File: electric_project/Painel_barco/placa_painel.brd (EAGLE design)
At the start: 60 x 100 mm, 15 parts, among them IC1 7805TV

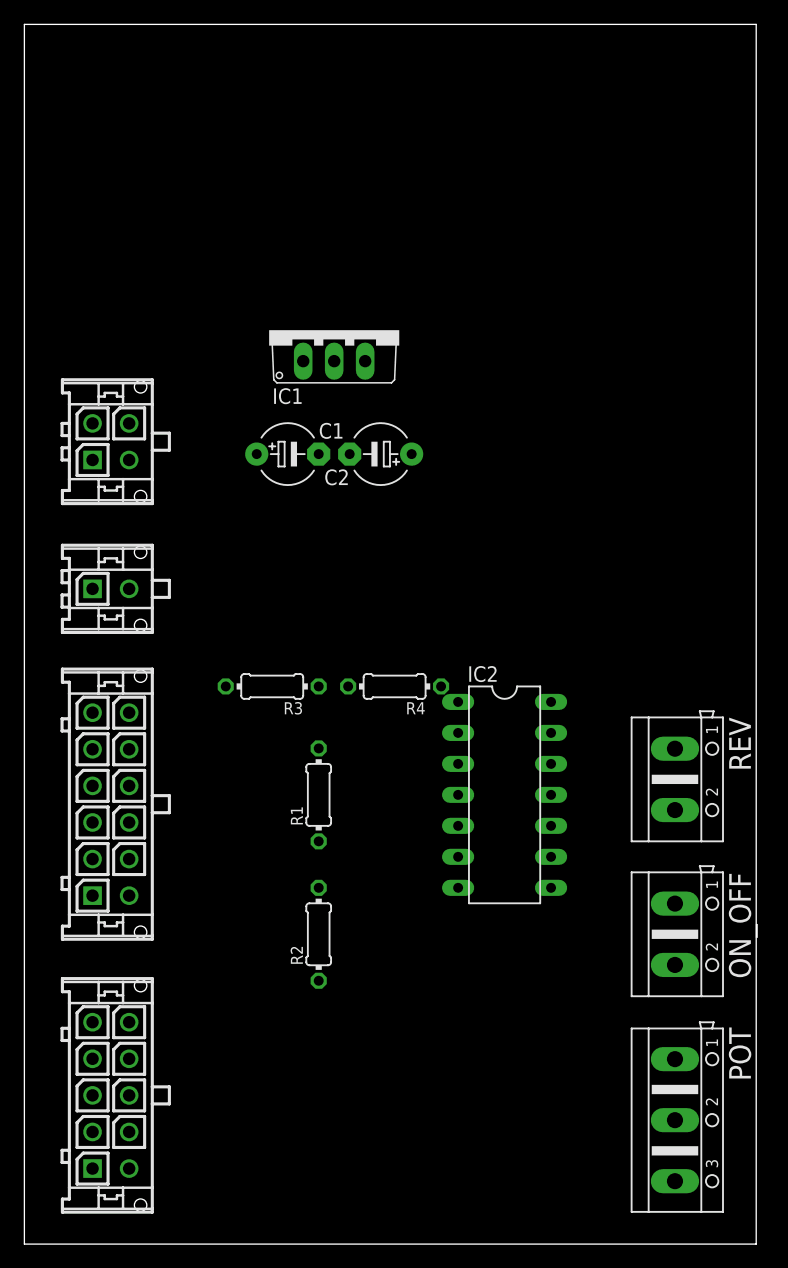
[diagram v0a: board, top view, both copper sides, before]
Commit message: up
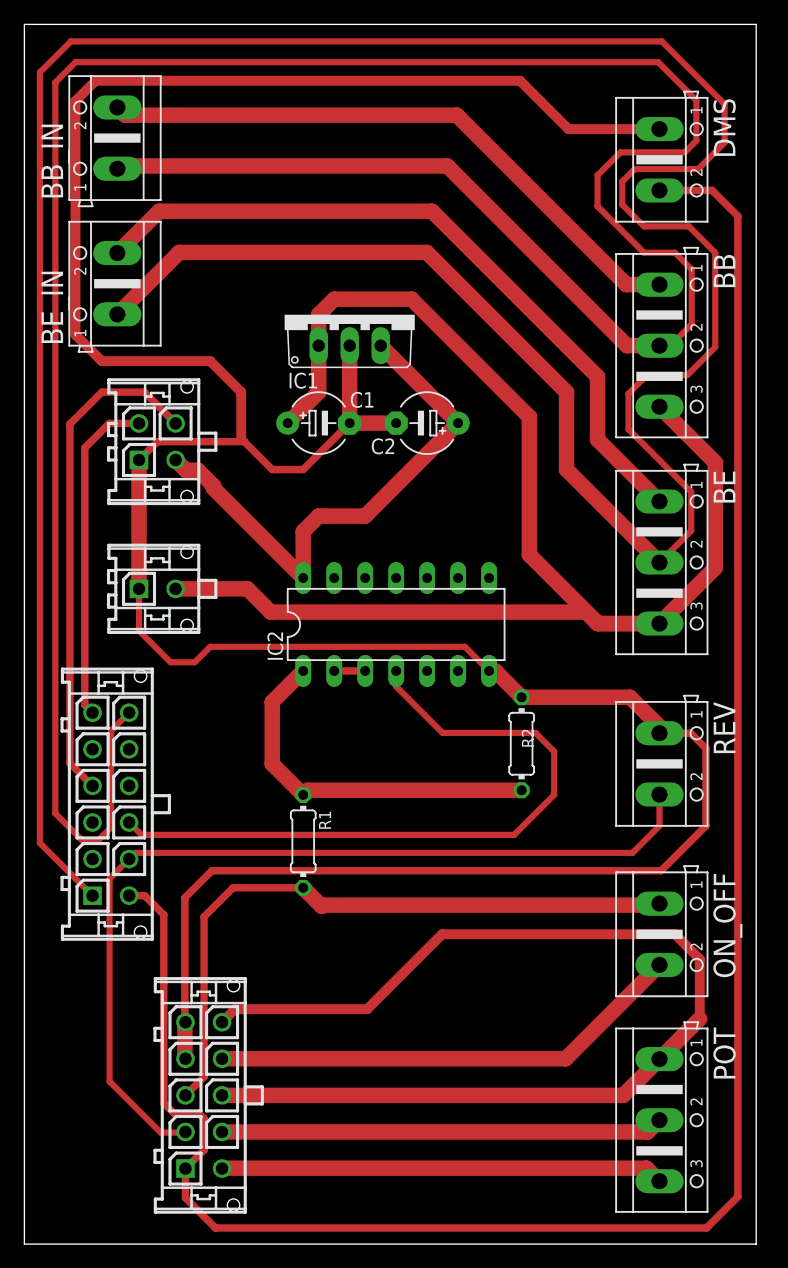
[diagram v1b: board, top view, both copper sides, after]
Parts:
- removed R3, R4: (no value), rcl:0204/7
- removed X2: (no value), con-molex-micro-fit-3_0:43045-1012
- added BB, BE: (no value), con-ptr500:AK500/3
- added BB_IN, BE_IN, DMS: (no value), con-ptr500:AK500/2
- added MOTOR_CON: (no value), con-molex-micro-fit-3_0:43045-1012
- moved R2 22.8 mm to (40.8, 41.0), turned to 270 degrees
- moved IC2 16.6 mm to (30.5, 50.8), turned to 0 degrees
- moved C2 4.58 mm to (33.0, 67.3)
- moved R1 4.02 mm to (22.9, 33.0), turned to 270 degrees
- moved X3 3.81 mm to (9.40, 53.7)
- moved X7 3.81 mm to (9.40, 65.8)
- moved C1 3.59 mm to (24.1, 67.3)
- moved IC1 1.80 mm to (26.7, 76.2)
- moved REV 1.80 mm to (52.1, 39.4)
- moved ON_OFF 1.27 mm to (52.1, 25.4)
- moved POT 1.27 mm to (52.1, 10.2)
- renumbered X1 to TELE_CON
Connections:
- removed net BB_IN: TELE_CON.P$12
- removed net BE_IN: TELE_CON.P$1
- removed net DMS_IN: TELE_CON.P$7
- removed net N$8: R3.1, R4.2
- new net BB_AUTO: BB.1, BB_IN.2
- new net BB_RET: BB.2, BB_IN.1, TELE_CON.P$12
- new net BE_AUTO: BE.1, BE_IN.2
- new net BE_RET: BE.2, BE_IN.1, TELE_CON.P$1
- new net WHITE_DMS: DMS.2, MOTOR_CON.P$1, TELE_CON.P$7
- net 21: now also X7.P$4; no longer X7.P$3
- net 22: now also X7.P$2; no longer X7.P$4
- net BLACK_GND: now also MOTOR_CON.P$10, MOTOR_CON.P$8; no longer X2.P$10, X2.P$8
- net BLUE_5V: now also MOTOR_CON.P$6; no longer X2.P$6
- net BROWN_REVERSE: now also MOTOR_CON.P$2; no longer X2.P$2
- net GND: now also DMS.1, MOTOR_CON.P$4, MOTOR_CON.P$5; no longer R4.1, X2.P$4, X2.P$5
- net PURP_45V_ONOFF_BACK: now also MOTOR_CON.P$3; no longer R3.2, X2.P$3
- net RED_ONOFF_45V_PH: now also MOTOR_CON.P$9; no longer X2.P$9
- net VCC_12: now also BB.3, BE.3
- net VCC_5V: now also X7.P$3; no longer X7.P$2
- net WHITE_CRUISE: no longer X2.P$1
- net YEL_POT_MEASURE: now also MOTOR_CON.P$7; no longer X2.P$7
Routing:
- net GND: track 0.00 -> 250.3 mm
- net BE_RET: track 0.00 -> 246.9 mm
- net BB_RET: track 0.00 -> 213.9 mm
- net WHITE_DMS: track 0.00 -> 165.0 mm
- net VCC_12: track 0.00 -> 118.5 mm
- net BLACK_GND: track 0.00 -> 89.7 mm
- net BROWN_REVERSE: track 0.00 -> 74.1 mm
- net BE_AUTO: track 0.00 -> 58.7 mm
- net ONOFF_MOTOR: track 0.00 -> 56.6 mm
- net PURP_45V_ONOFF_BACK: track 0.00 -> 54.4 mm
- net BB_AUTO: track 0.00 -> 50.5 mm
- net VCC_5V: track 0.00 -> 43.8 mm
- net 21: track 0.00 -> 41.2 mm
- net RED_ONOFF_45V_PH: track 0.00 -> 39.0 mm
- net BLUE_5V: track 0.00 -> 36.3 mm
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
